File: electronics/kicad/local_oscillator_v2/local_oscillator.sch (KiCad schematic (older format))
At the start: 31 parts, among them P1 TestPoint:TestPoint_Pad_1.5x1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, P2 TestPoint:TestPoint_Pad_1.5x1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, P3 TestPoint:TestPoint_Pad_1.5x1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, P4 TestPoint:TestPoint_Pad_1.5x1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, P5 TestPoint:TestPoint_Pad_1.5x1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, P6 TestPoint:TestPoint_Pad_1.5x1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, P7 TestPoint:TestPoint_Pad_1.5x1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, P8 TestPoint:TestPoint_Pad_1.5x1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, Q1 BSS138, Q2 BSS138, U1 CE3520K3

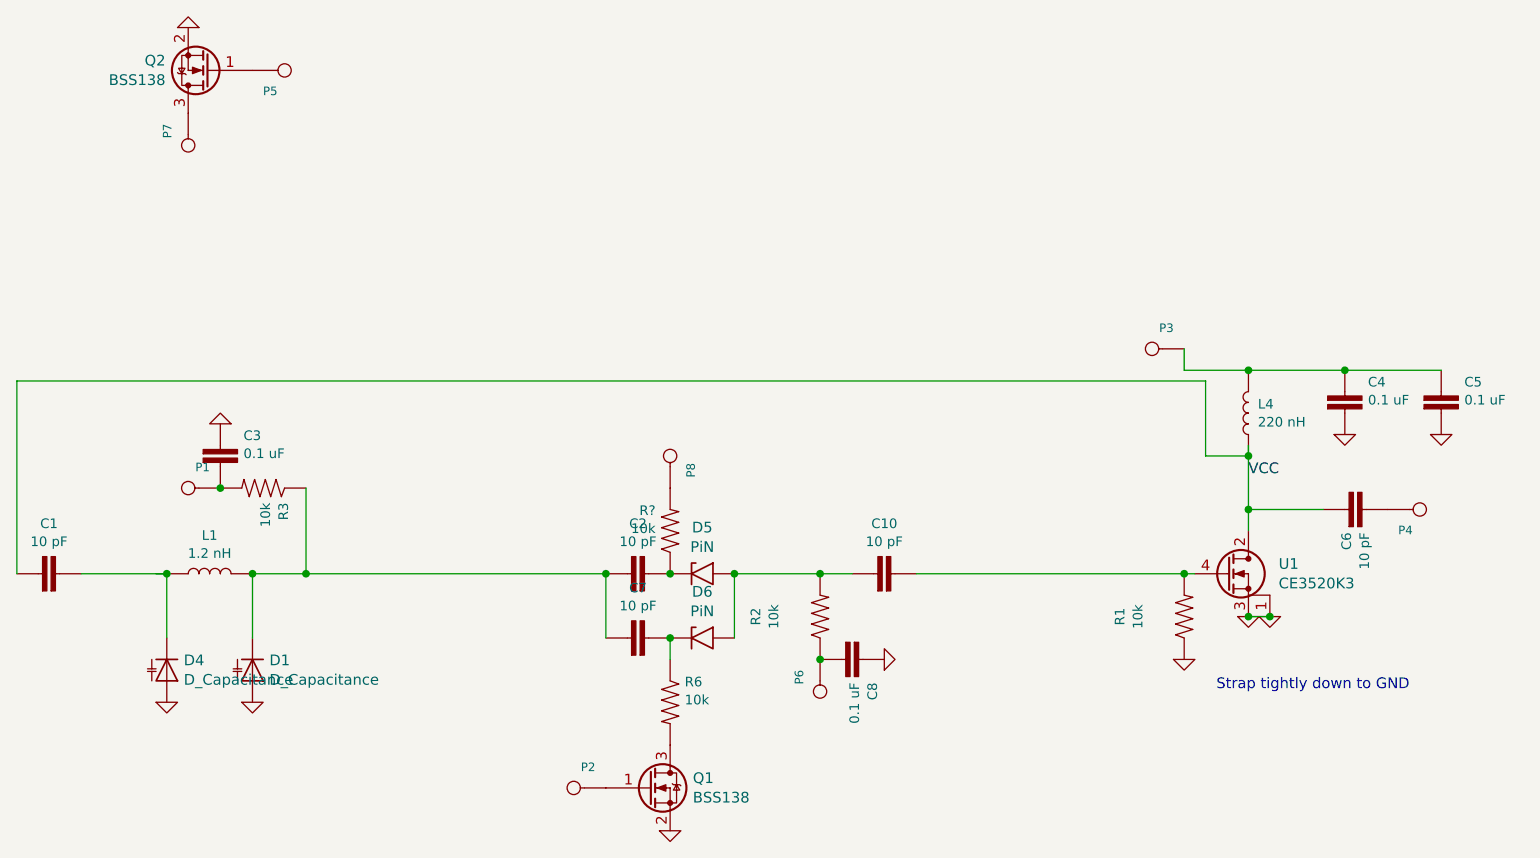
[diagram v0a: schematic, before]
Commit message: 4-pole LO
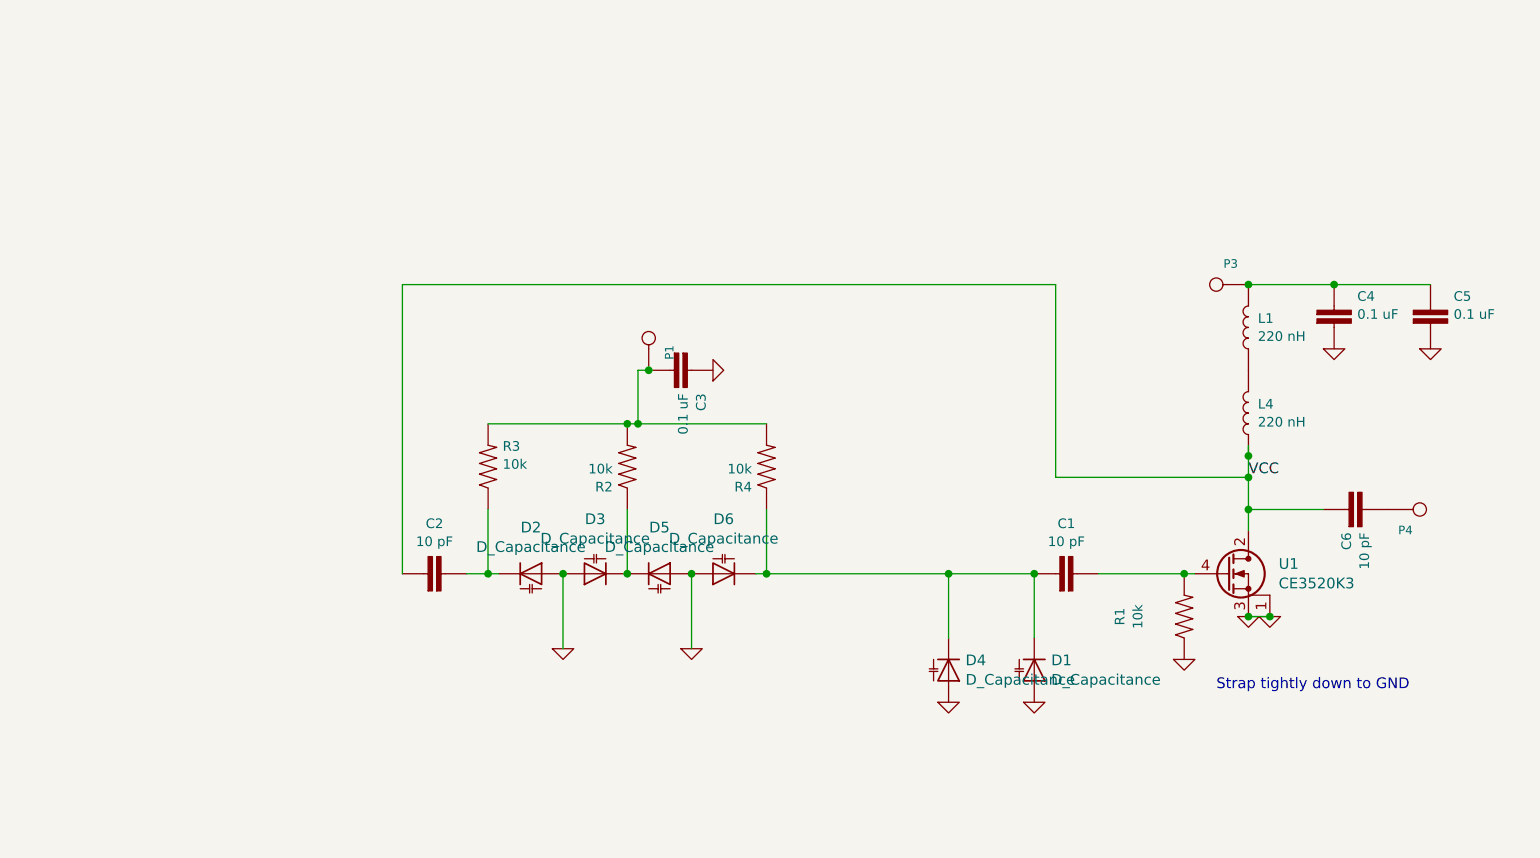
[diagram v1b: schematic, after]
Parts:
- removed C10, C7: 10 pF, 0402, symbol SparkFun-Capacitors:6PF-0402-50V-0.5%
- removed C8: 0.1 uF, 0603, symbol SparkFun-Capacitors:4.7UF0603
- removed D5, D6: PiN, Diode_SMD:D_SOD-523, symbol Diode:1.5KExxA
- removed P2, P5, P6, P7: TestPoint:TestPoint_Pad_1.5x1.5mm, TestPoint:TestPoint_Pad_1.5x1.5mm, symbol conn:CONN_1
- removed P8: TestPoint:TestPoint_Pad_1.5x1.5mm, TestPoint:TestPoint_Pad_D1.0mm, symbol conn:CONN_1
- removed Q1, Q2: BSS138, Package_TO_SOT_SMD:SOT-23, symbol Transistor_FET:BSS138
- removed R6, R?: 10k, 0402, symbol SparkFun-Resistors:RESISTOR0402
- added D2, D3, D5, D6: D_Capacitance, Diode_SMD:D_SOD-523, symbol Device:D_Capacitance
- added R4: 10k, 0402, symbol SparkFun-Resistors:RESISTOR0402
- L1: value 1.2 nH -> 220 nH
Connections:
- wire segments 27 -> 31
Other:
- moved on the sheet: C1, C4, C5, D1, D4, P3, R3

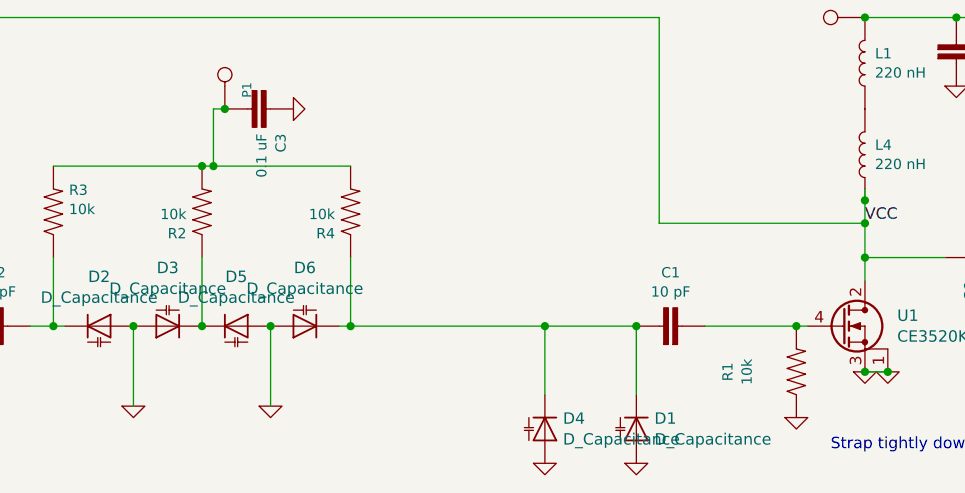
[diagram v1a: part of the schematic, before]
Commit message: SPICE
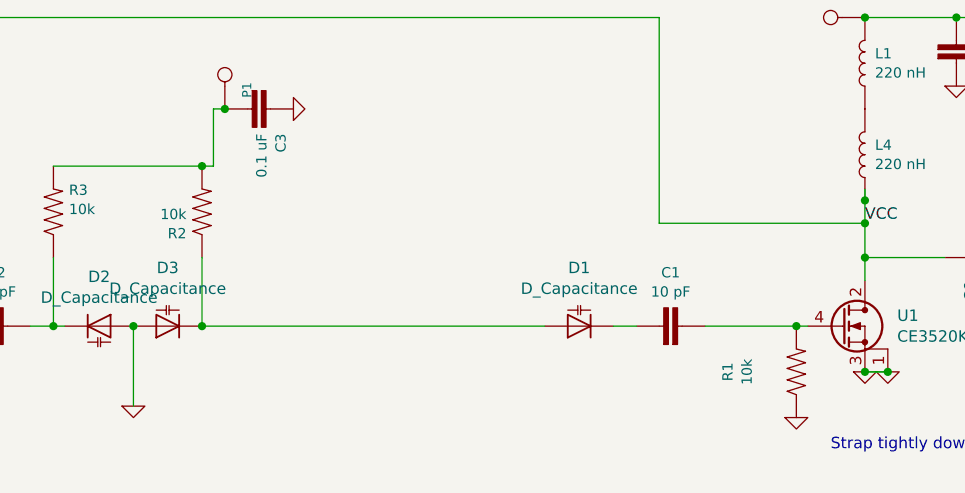
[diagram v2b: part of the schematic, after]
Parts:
- removed D4, D5, D6: D_Capacitance, Diode_SMD:D_SOD-523, symbol Device:D_Capacitance
- removed R4: 10k, 0402, symbol SparkFun-Resistors:RESISTOR0402
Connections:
- wire segments 31 -> 25
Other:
- moved on the sheet: D1
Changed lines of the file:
@@
-$EndComp
-$Comp
-L power:GND #PWR0107
-U 1 1 5EE0E867
-P 6900 5200
-F 0 "#PWR0107" H 6900 5200 30  0001 C CNN
-F 1 "GND" H 6900 5130 30  0001 C CNN
-F 2 "" H 6900 5200 50  0001 C CNN
-F 3 "" H 6900 5200 50  0001 C CNN
-	1    6900 5200
-	1    0    0    -1
-$EndComp
-$Comp
-L Device:D_Capacitance D4
-U 1 1 5EE0E0B0
-P 6900 5050
-F 0 "D4" V 6854 5129 50  0000 L CNN
-F 1 "D_Capacitance" V 6945 5129 50  0000 L CNN
-F 2 "Diode_SMD:D_SOD-523" H 6900 5050 50  0001 C CNN
-F 3 "~" H 6900 5050 50  0001 C CNN
-	1    6900 5050
-	0    1    1    0
-$EndComp
-$Comp
-L power:GND #PWR0106
-U 1 1 5EE0BB79
-P 7300 5200
-F 0 "#PWR0106" H 7300 5200 30  0001 C CNN
-F 1 "GND" H 7300 5130 30  0001 C CNN
-F 2 "" H 7300 5200 50  0001 C CNN
-F 3 "" H 7300 5200 50  0001 C CNN
-	1    7300 5200
-	1    0    0    -1
 $EndComp
 $Comp
 L Device:D_Capacitance D1
 U 1 1 5ED19292
-P 7300 5050
-F 0 "D1" V 7254 5129 50  0000 L CNN
-F 1 "D_Capacitance" V 7345 5129 50  0000 L CNN
-F 2 "Diode_SMD:D_SOD-523" H 7300 5050 50  0001 C CNN
-F 3 "~" H 7300 5050 50  0001 C CNN
-	1    7300 5050
-	0    1    1    0
-$EndComp
-Wire Wire Line
-	7300 4900 7300 4600
-Wire Wire Line
-	6900 4900 6900 4600
+P 7050 4600
+F 0 "D1" H 7050 4345 50  0000 C CNN
+F 1 "D_Capacitance" H 7050 4436 50  0000 C CNN
+F 2 "Diode_SMD:D_SOD-523" H 7050 4600 50  0001 C CNN
+F 3 "~" H 7050 4600 50  0001 C CNN
+	1    7050 4600
+	-1   0    0    1
+$EndComp
 $Comp
 L SparkFun-Resistors:RESISTOR0402 R3
@@
 	-1   0    0    1
 $EndComp
-Wire Wire Line
-	6900 4600 7300 4600
-Connection ~ 7300 4600
 $Comp
 L SparkFun-Capacitors:6PF-0402-50V-0.5% C2
@@
 	-1   0    0    1
 $EndComp
-$Comp
-L Device:D_Capacitance D5
-U 1 1 5F005E53
-P 5550 4600
-F 0 "D5" H 5550 4816 50  0000 C CNN
-F 1 "D_Capacitance" H 5550 4725 50  0000 C CNN
-F 2 "Diode_SMD:D_SOD-523" H 5550 4600 50  0001 C CNN
-F 3 "~" H 5550 4600 50  0001 C CNN
-	1    5550 4600
-	1    0    0    -1
-$EndComp
-$Comp
-L Device:D_Capacitance D6
-U 1 1 5F007895
-P 5850 4600
-F 0 "D6" H 5850 4345 50  0000 C CNN
-F 1 "D_Capacitance" H 5850 4436 50  0000 C CNN
-F 2 "Diode_SMD:D_SOD-523" H 5850 4600 50  0001 C CNN
-F 3 "~" H 5850 4600 50  0001 C CNN
-	1    5850 4600
-	-1   0    0    1
-$EndComp
-Wire Wire Line
-	6000 4600 6050 4600
-Connection ~ 6900 4600
 Wire Wire Line
 	4800 4600 4750 4600
@@
 	5100 4600 5100 4950
 Connection ~ 5100 4600
-Wire Wire Line
-	5700 4600 5700 4950
-Connection ~ 5700 4600
-$Comp
-L power:GND #PWR0108
-U 1 1 5F009480
-P 5700 4950
-F 0 "#PWR0108" H 5700 4950 30  0001 C CNN
-F 1 "GND" H 5700 4880 30  0001 C CNN
-F 2 "" H 5700 4950 50  0001 C CNN
-F 3 "" H 5700 4950 50  0001 C CNN
-	1    5700 4950
-	1    0    0    -1
-$EndComp
 $Comp
 L power:GND #PWR0110
@@
 	0    -1   -1   0
 $EndComp
-$Comp
-L SparkFun-Resistors:RESISTOR0402 R4
-U 1 1 5F02BE58
-P 6050 4100
-F 0 "R4" V 5955 4168 45  0000 L CNN
-F 1 "10k" V 6039 4168 45  0000 L CNN
-F 2 "0402" H 6050 4250 20  0001 C CNN
-F 3 "" H 6050 4100 60  0001 C CNN
-F 4 " " V 6134 4168 60  0000 L CNN "Field4"
-	1    6050 4100
-	0    -1   -1   0
-$EndComp
 Wire Wire Line
 	5450 3900 5450 3650
-Wire Wire Line
-	5450 3900 6050 3900
-Connection ~ 5450 3900
 Wire Wire Line
 	5450 3900 5400 3900
@@
 Wire Wire Line
 	5400 4600 5400 4300
-Connection ~ 5400 4600
-Wire Wire Line
-	6050 4300 6050 4600
-Connection ~ 6050 4600
-Wire Wire Line
-	6050 4600 6900 4600
 Wire Wire Line
 	4750 4300 4750 4600
@@
 Wire Wire Line
 	8300 4150 8300 4300
+Wire Wire Line
+	5400 4600 6900 4600
+Connection ~ 5400 4600
+Wire Wire Line
+	7200 4600 7300 4600
 $EndSCHEMATC

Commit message: SVG import improvements
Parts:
- P1: value TestPoint:TestPoint_Pad_1.5x1.5mm -> T
- P3, P4: value TestPoint:TestPoint_Pad_1.5x1.5mm -> a
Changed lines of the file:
@@
 P 9100 4300
 F 0 "P4" H 9033 4203 40  0000 C CNN
-F 1 "TestPoint:TestPoint_Pad_1.5x1.5mm" H 9050 4340 30  0001 C CNN
+F 1 "a" H 9050 4340 30  0001 C CNN
 F 2 "TestPoint:TestPoint_Pad_1.5x1.5mm" H 9100 4300 50  0001 C CNN
 F 3 "" H 9100 4300 50  0001 C CNN
@@
 P 8150 3250
 F 0 "P3" H 8083 3153 40  0000 C CNN
-F 1 "TestPoint:TestPoint_Pad_1.5x1.5mm" H 8100 3290 30  0001 C CNN
+F 1 "a" H 8100 3290 30  0001 C CNN
 F 2 "TestPoint:TestPoint_Pad_1.5x1.5mm" H 8150 3250 50  0001 C CNN
 F 3 "" H 8150 3250 50  0001 C CNN
@@
 P 5500 3500
 F 0 "P1" H 5433 3403 40  0000 C CNN
-F 1 "TestPoint:TestPoint_Pad_1.5x1.5mm" H 5450 3540 30  0001 C CNN
+F 1 "T" H 5450 3540 30  0001 C CNN
 F 2 "TestPoint:TestPoint_Pad_1.5x1.5mm" H 5500 3500 50  0001 C CNN
 F 3 "" H 5500 3500 50  0001 C CNN
